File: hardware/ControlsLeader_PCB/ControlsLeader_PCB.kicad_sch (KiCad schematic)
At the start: 13 parts, among them J1 CarCANConnector_Out, J2 PeripheralCAN_out, J3 CarCANConnector_In, J4 PeripheralCAN_in, J6 Conn_2Rows-09Pins, J7 Dash_LSOM_PWR, J8 Conn_2Rows-09Pins, U2 LeaderSOM

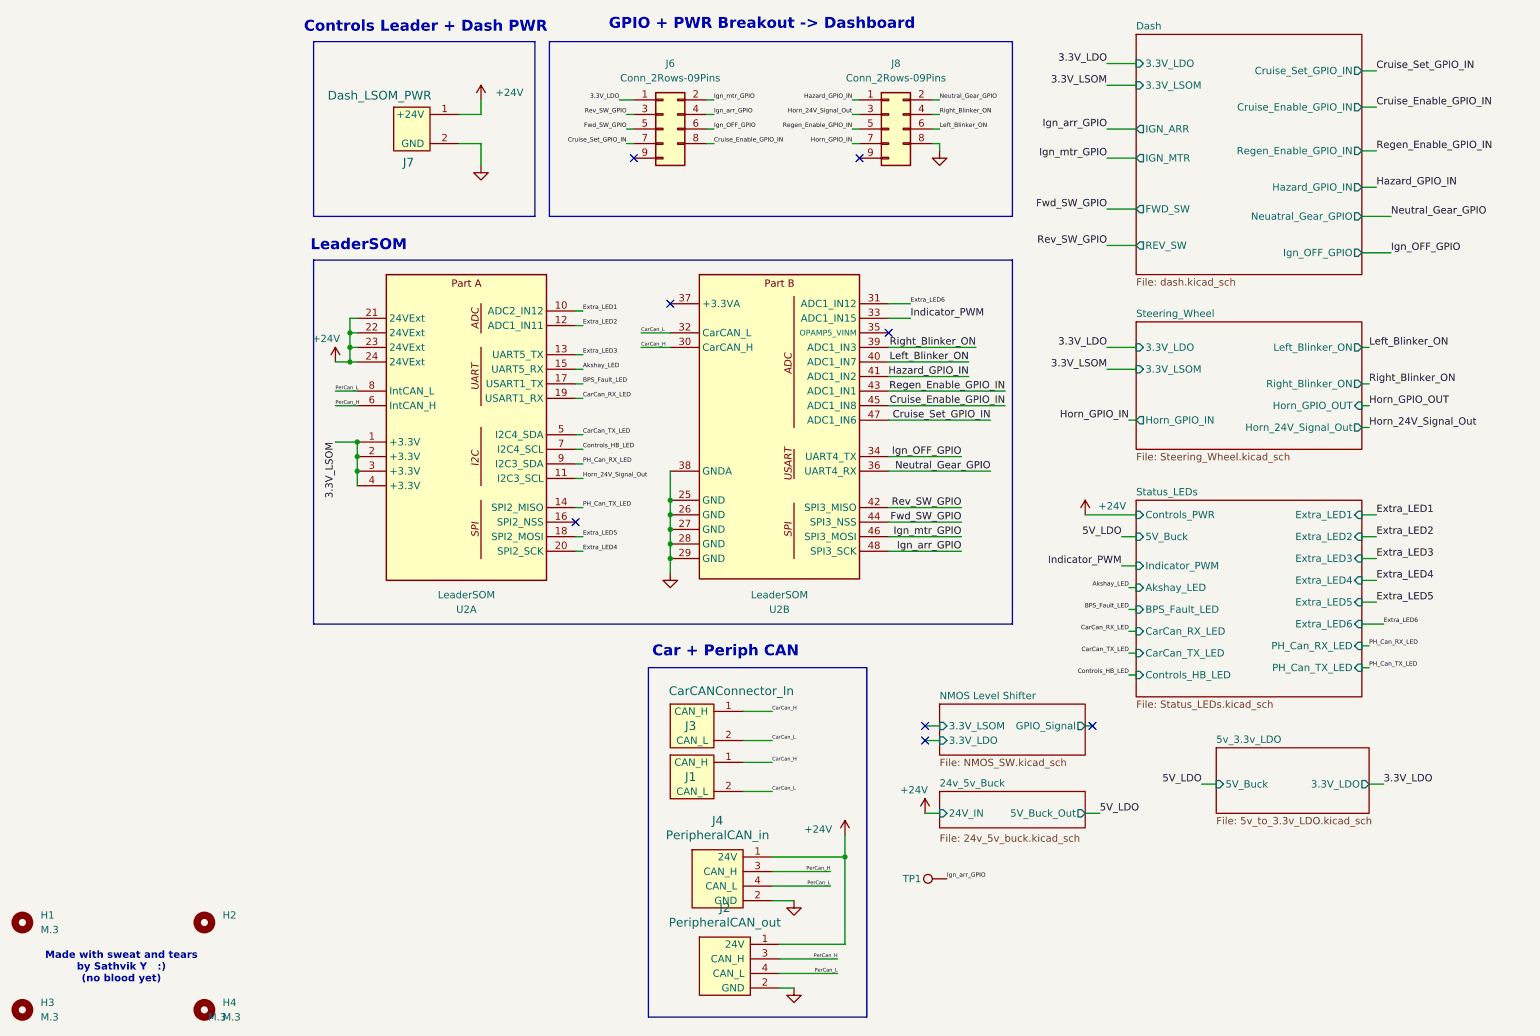
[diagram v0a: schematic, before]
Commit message: Ready for final review
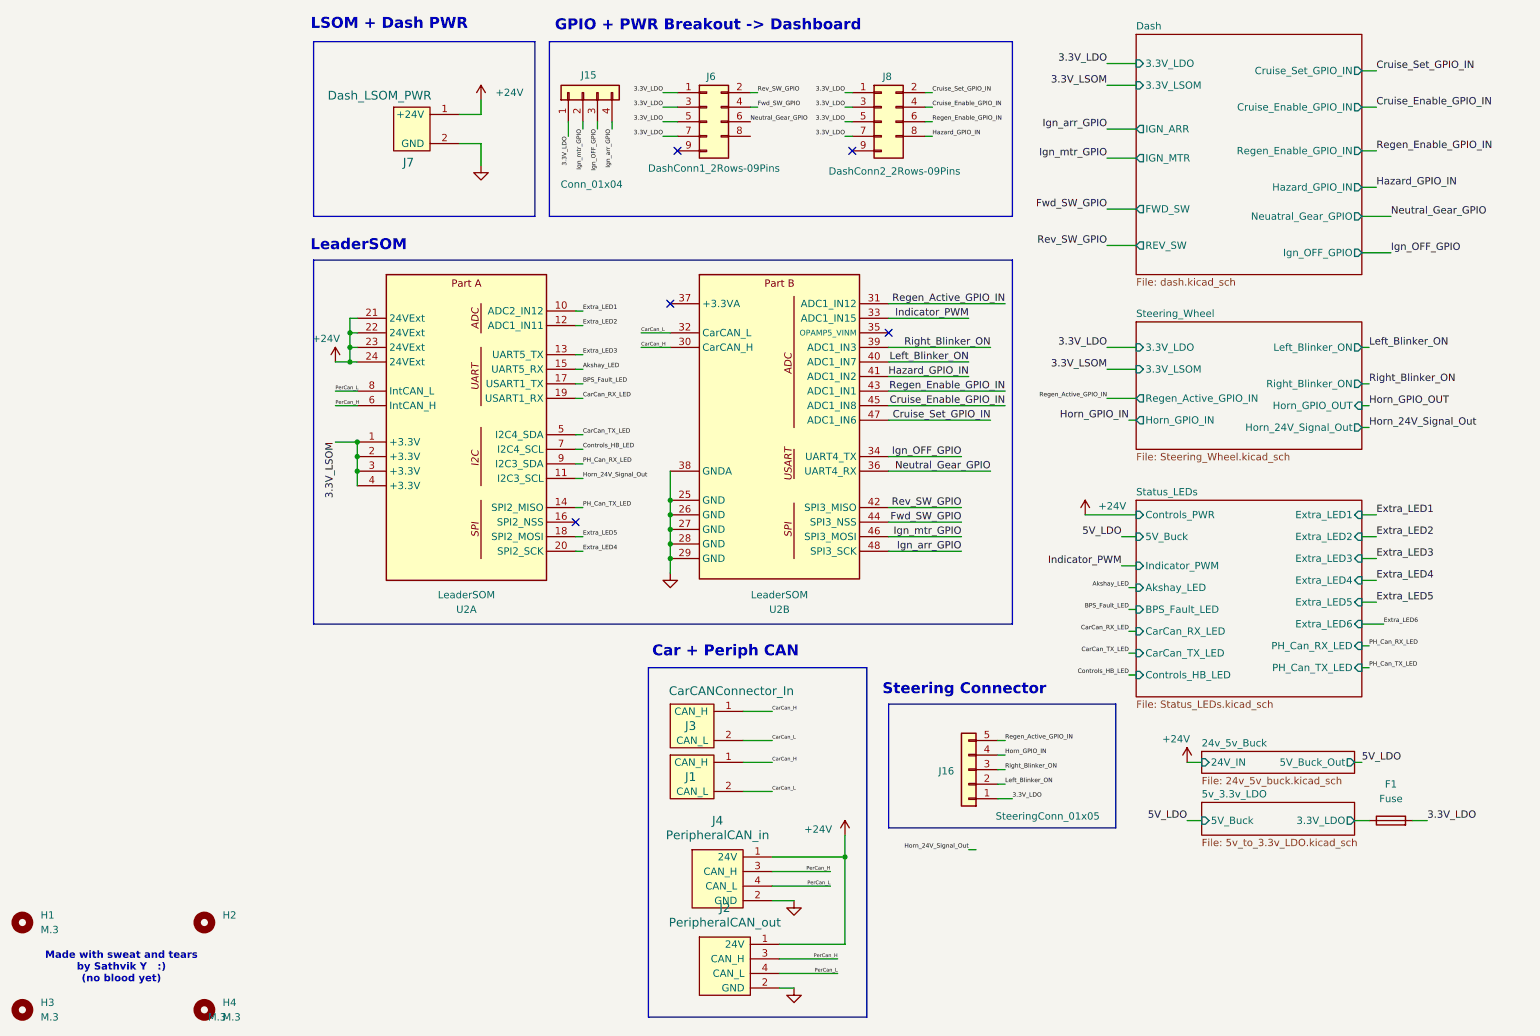
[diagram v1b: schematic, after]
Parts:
- removed TP1: TestPoint, TestPoint:TestPoint_Pad_1.0x1.0mm, symbol Connector:TestPoint
- added F1: Fuse, Fuse:Fuseholder_Blade_Mini_Keystone_3568, symbol Device:Fuse
- added J15: Conn_01x04, Connector_Molex:Molex_Nano-Fit_105313-xx04_1x04_P2.50mm_Horizontal, symbol Connector_Generic:Conn_01x04
- added J16: SteeringConn_01x05, Connector_Molex:Molex_Nano-Fit_105313-xx05_1x05_P2.50mm_Horizontal, symbol Connector_Generic:Conn_01x05
- J6: value Conn_2Rows-09Pins -> DashConn1_2Rows-09Pins
- J8: value Conn_2Rows-09Pins -> DashConn2_2Rows-09Pins
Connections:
- net 3.3V_LDO: now also J6.3 (Pin_3), J6.5 (Pin_5), J6.7 (Pin_7), J8.1 (Pin_1), J8.3 (Pin_3), J8.5 (Pin_5), J8.7 (Pin_7), F1.2, J15.1 (Pin_1), J16.1 (Pin_1)
- net Cruise_Enable_GPIO_IN: now also J8.4 (Pin_4); no longer J6.8 (Pin_8)
- net Cruise_Set_GPIO_IN: now also J8.2 (Pin_2); no longer J6.7 (Pin_7)
- net Extra_LED6: no longer U2.31 (ADC1_IN12)
- net Fwd_SW_GPIO: now also J6.4 (Pin_4); no longer J6.5 (Pin_5)
- net GND: no longer J8.8 (Pin_8)
- net Hazard_GPIO_IN: now also J8.8 (Pin_8); no longer J8.1 (Pin_1)
- net Horn_24V_Signal_Out: no longer J8.3 (Pin_3)
- net Horn_GPIO_IN: now also J16.4 (Pin_4); no longer J8.7 (Pin_7)
- net Ign_OFF_GPIO: now also J15.3 (Pin_3); no longer J6.6 (Pin_6)
- net Ign_arr_GPIO: now also J15.4 (Pin_4); no longer J6.4 (Pin_4)
- net Ign_mtr_GPIO: now also J15.2 (Pin_2); no longer J6.2 (Pin_2)
- net Left_Blinker_ON: now also J16.2 (Pin_2); no longer J8.6 (Pin_6)
- net Neutral_Gear_GPIO: now also J6.6 (Pin_6); no longer J8.2 (Pin_2)
- net Regen_Enable_GPIO_IN: now also J8.6 (Pin_6); no longer J8.5 (Pin_5)
- net Rev_SW_GPIO: now also J6.2 (Pin_2); no longer J6.3 (Pin_3)
- net Right_Blinker_ON: now also J16.3 (Pin_3); no longer J8.4 (Pin_4)
- new net 5v_3.3v_LDO/3.3V_LDO: F1.1
- new net Regen_Active_GPIO_IN: J16.5 (Pin_5), U2.31 (ADC1_IN12)
- no-connect marks 8 -> 5
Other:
- removed sheet NMOS Level Shifter
- sheet Steering_Wheel ports: added Regen_Active_GPIO_IN; removed none
- note added: "LSOM + Dash PWR"
- note added: "Steering Connector"
- note removed: "Controls Leader + Dash PWR"
